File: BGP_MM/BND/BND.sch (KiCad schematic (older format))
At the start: 4 parts, among them J1 Conn_01x02, J2 Conn_01x03, P1 CONN_01X02

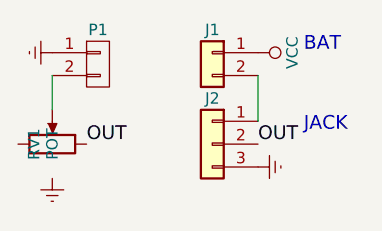
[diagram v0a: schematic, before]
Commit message: MM Refactoring
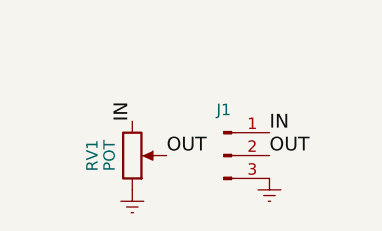
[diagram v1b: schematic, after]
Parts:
- removed J1: Conn_01x02, Terminal_Blocks:TerminalBlock_Pheonix_MPT-2.54mm_2pol, symbol Conn_01x02
- removed J2: Conn_01x03, Terminal_Blocks:TerminalBlock_Pheonix_MPT-2.54mm_3pol, symbol Conn_01x03
- removed P1: CONN_01X02, Connectors_JST:JST_PH_B2B-PH-K_02x2.00mm_Straight, symbol CONN_01X02
- added J1: Conn_01x03_Male, Pin_Headers:Pin_Header_Straight_1x03_Pitch2.54mm, symbol Conn_01x03_Male
- RV1: footprint LIBS:Potentiometer_Alpha_RV16 -> (none)
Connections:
- net Earth: now also RV1.1, J1.3 (Pin_3)
- net OUT: now also RV1.2, J1.2 (Pin_2); no longer RV1.1
- net IN: now reaches RV1.3
- net IN: now also J1.1 (Pin_1)
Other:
- note removed: "BAT"
- note removed: "JACK"
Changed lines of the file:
@@
 LIBS:switches
 LIBS:relays
+LIBS:motors
 LIBS:transistors
 LIBS:conn
@@
 $EndDescr
 $Comp
-L Conn_01x02 J1
-U 1 1 5AE4EB86
-P 6500 3450
-F 0 "J1" H 6500 3550 50  0000 C CNN
-F 1 "Conn_01x02" H 6500 3250 50  0001 C CNN
-F 2 "Terminal_Blocks:TerminalBlock_Pheonix_MPT-2.54mm_2pol" H 6500 3450 50  0001 C CNN
-F 3 "" H 6500 3450 50  0001 C CNN
-	1    6500 3450
-	-1   0    0    -1
+L POT RV1
+U 1 1 5B1AF2D3
+P 6150 3900
+F 0 "RV1" V 5975 3900 50  0000 C CNN
+F 1 "POT" V 6050 3900 50  0000 C CNN
+F 2 "" H 6150 3900 50  0001 C CNN
+F 3 "" H 6150 3900 50  0001 C CNN
+	1    6150 3900
+	1    0    0    1
 $EndComp
-$Comp
-L Conn_01x03 J2
-U 1 1 5AE533B1
-P 6500 3850
-F 0 "J2" H 6500 4050 50  0000 C CNN
-F 1 "Conn_01x03" H 6500 3650 50  0001 C CNN
-F 2 "Terminal_Blocks:TerminalBlock_Pheonix_MPT-2.54mm_3pol" H 6500 3850 50  0001 C CNN
-F 3 "" H 6500 3850 50  0001 C CNN
-	1    6500 3850
-	-1   0    0    -1
-$EndComp
+Text Label 6150 3750 1    60   ~ 0
+IN
+Text Label 6300 3900 0    60   ~ 0
+OUT
 $Comp
 L Earth #PWR01
-U 1 1 5B063927
-P 6700 3950
-F 0 "#PWR01" H 6700 3700 50  0001 C CNN
-F 1 "Earth" H 6700 3800 50  0001 C CNN
-F 2 "" H 6700 3950 50  0001 C CNN
-F 3 "" H 6700 3950 50  0001 C CNN
-	1    6700 3950
-	0    -1   -1   0
-$EndComp
-Text Label 6700 3850 0    60   ~ 0
-OUT
-$Comp
-L VCC #PWR02
-U 1 1 5B063954
-P 6700 3450
-F 0 "#PWR02" H 6700 3300 50  0001 C CNN
-F 1 "VCC" H 6700 3600 50  0000 C CNN
-F 2 "" H 6700 3450 50  0000 C CNN
-F 3 "" H 6700 3450 50  0000 C CNN
-	1    6700 3450
-	0    1    1    0
-$EndComp
-Text Notes 6900 3450 0    60   ~ 0
-BAT
-Text Notes 6900 3800 0    60   ~ 0
-JACK
-Wire Wire Line
-	6700 3750 6700 3550
-$Comp
-L CONN_01X02 P1
-U 1 1 5B19CB22
-P 6000 3500
-F 0 "P1" H 6000 3650 50  0000 C CNN
-F 1 "CONN_01X02" V 6100 3500 50  0001 C CNN
-F 2 "Connectors_JST:JST_PH_B2B-PH-K_02x2.00mm_Straight" H 6000 3500 50  0001 C CNN
-F 3 "" H 6000 3500 50  0000 C CNN
-	1    6000 3500
+U 1 1 5B1AF2FA
+P 6150 4050
+F 0 "#PWR01" H 6150 3800 50  0001 C CNN
+F 1 "Earth" H 6150 3900 50  0001 C CNN
+F 2 "" H 6150 4050 50  0001 C CNN
+F 3 "" H 6150 4050 50  0001 C CNN
+	1    6150 4050
 	1    0    0    -1
 $EndComp
 $Comp
-L Earth #PWR03
-U 1 1 5B19CBB0
-P 5800 3450
-F 0 "#PWR03" H 5800 3200 50  0001 C CNN
-F 1 "Earth" H 5800 3300 50  0001 C CNN
-F 2 "" H 5800 3450 50  0000 C CNN
-F 3 "" H 5800 3450 50  0000 C CNN
-	1    5800 3450
-	0    1    1    0
+L Conn_01x03_Male J1
+U 1 1 5B1AF310
+P 6550 3900
+F 0 "J1" H 6550 4100 50  0000 C CNN
+F 1 "Conn_01x03_Male" H 6550 3700 50  0001 C CNN
+F 2 "Pin_Headers:Pin_Header_Straight_1x03_Pitch2.54mm" H 6550 3900 50  0001 C CNN
+F 3 "" H 6550 3900 50  0001 C CNN
+	1    6550 3900
+	1    0    0    -1
 $EndComp
-$Comp
-L POT RV1
-U 1 1 5B19CBED
-P 5800 3850
-F 0 "RV1" H 5800 3770 50  0000 C CNN
-F 1 "POT" H 5800 3850 50  0000 C CNN
-F 2 "LIBS:Potentiometer_Alpha_RV16" H 5800 3850 50  0001 C CNN
-F 3 "" H 5800 3850 50  0000 C CNN
-	1    5800 3850
-	0    1    -1   0
-$EndComp
-Text Label 5950 3850 0    60   ~ 0
+Text Label 6750 3800 0    60   ~ 0
+IN
+Text Label 6750 3900 0    60   ~ 0
 OUT
 $Comp
-L Earth #PWR04
-U 1 1 5B19CC5B
-P 5800 4000
-F 0 "#PWR04" H 5800 3750 50  0001 C CNN
-F 1 "Earth" H 5800 3850 50  0001 C CNN
-F 2 "" H 5800 4000 50  0001 C CNN
-F 3 "" H 5800 4000 50  0001 C CNN
-	1    5800 4000
+L Earth #PWR02
+U 1 1 5B1AF35E
+P 6750 4000
+F 0 "#PWR02" H 6750 3750 50  0001 C CNN
+F 1 "Earth" H 6750 3850 50  0001 C CNN
+F 2 "" H 6750 4000 50  0001 C CNN
+F 3 "" H 6750 4000 50  0001 C CNN
+	1    6750 4000
 	1    0    0    -1
 $EndComp
-Wire Wire Line
-	5800 3700 5800 3550
 $EndSCHEMATC
